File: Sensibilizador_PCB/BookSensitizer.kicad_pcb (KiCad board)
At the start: 2 copper layers, 70 x 57 mm, 40 parts, among them J3 Conn_inputs, M1 Fan, Q1 IRF630, Q2 IRF630, Q3 IRF630, Q4 IRF630, Q5 SI2302, T1 MountingHole_3.2mm_M3, T2 MountingHole_3.2mm_M3, T3 MountingHole_3.2mm_M3, U1 LM5104M, U2 LM5104M

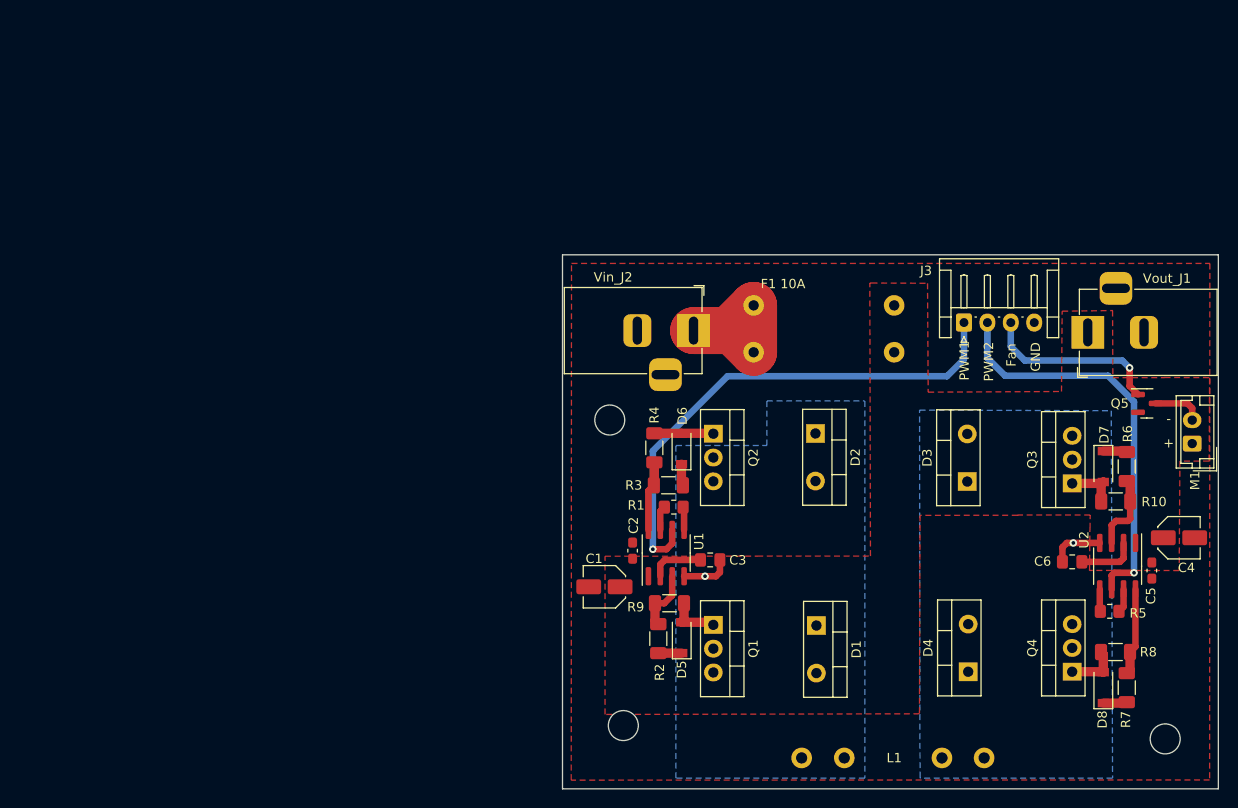
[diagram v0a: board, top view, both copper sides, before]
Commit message: mini arreglo para conectar una tierra
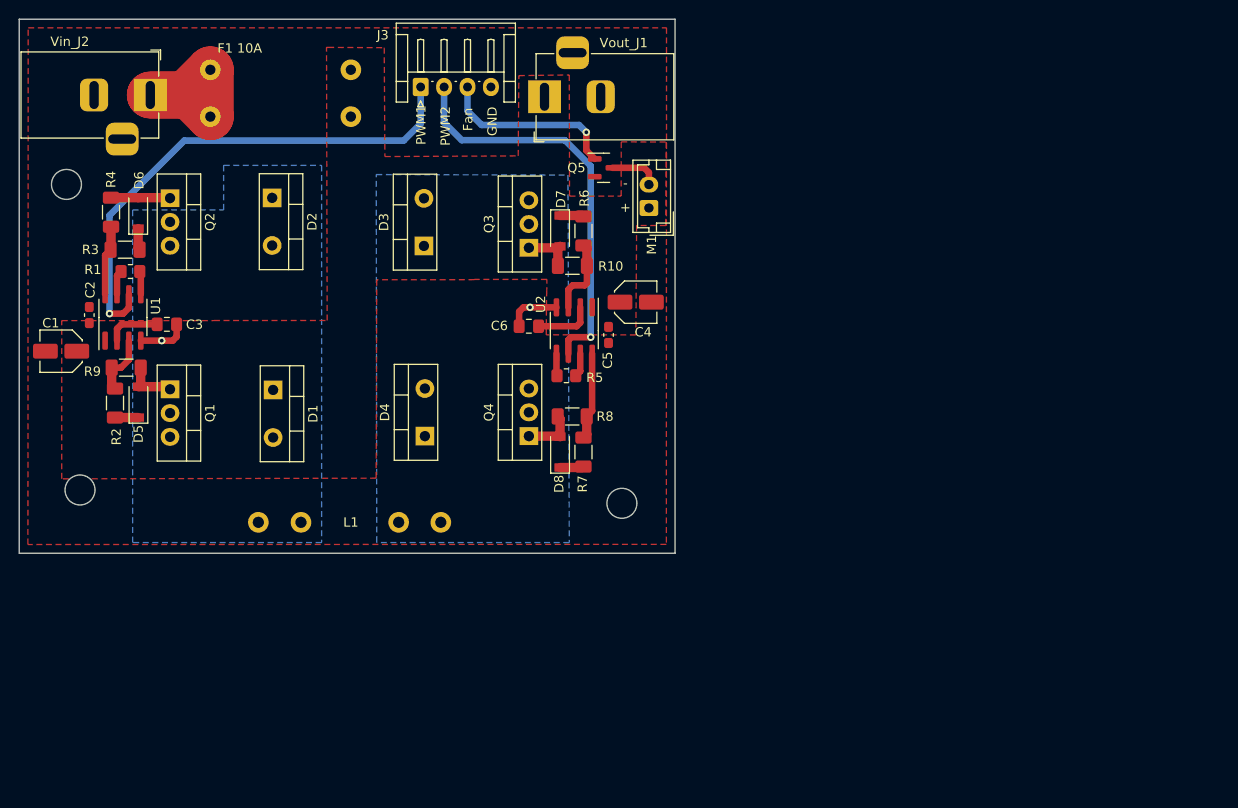
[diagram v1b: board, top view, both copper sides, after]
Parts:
- moved M1 63.2 mm to (118.1, 65.2)
- moved C2 63.2 mm to (58.4, 76.6)
- moved C3 63.2 mm to (66.7, 77.6)
- moved C5 63.2 mm to (113.8, 78.8)
- moved C6 63.2 mm to (105.3, 77.8)
- moved D1 63.2 mm to (78.0, 84.6)
- moved D2 63.2 mm to (77.9, 64.1)
- moved D7 63.2 mm to (108.6, 67.7)
- moved D8 63.2 mm to (108.6, 91.3)
- moved F1 10A 63.2 mm to (78.8, 53.0)
- moved J3 63.2 mm to (93.8, 52.3)
- moved Q1 63.2 mm to (67.0, 84.6)
- moved Q2 63.2 mm to (67.0, 64.2)
- moved Q3 63.2 mm to (105.3, 69.5)
- moved Q4 63.2 mm to (105.3, 89.6)
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
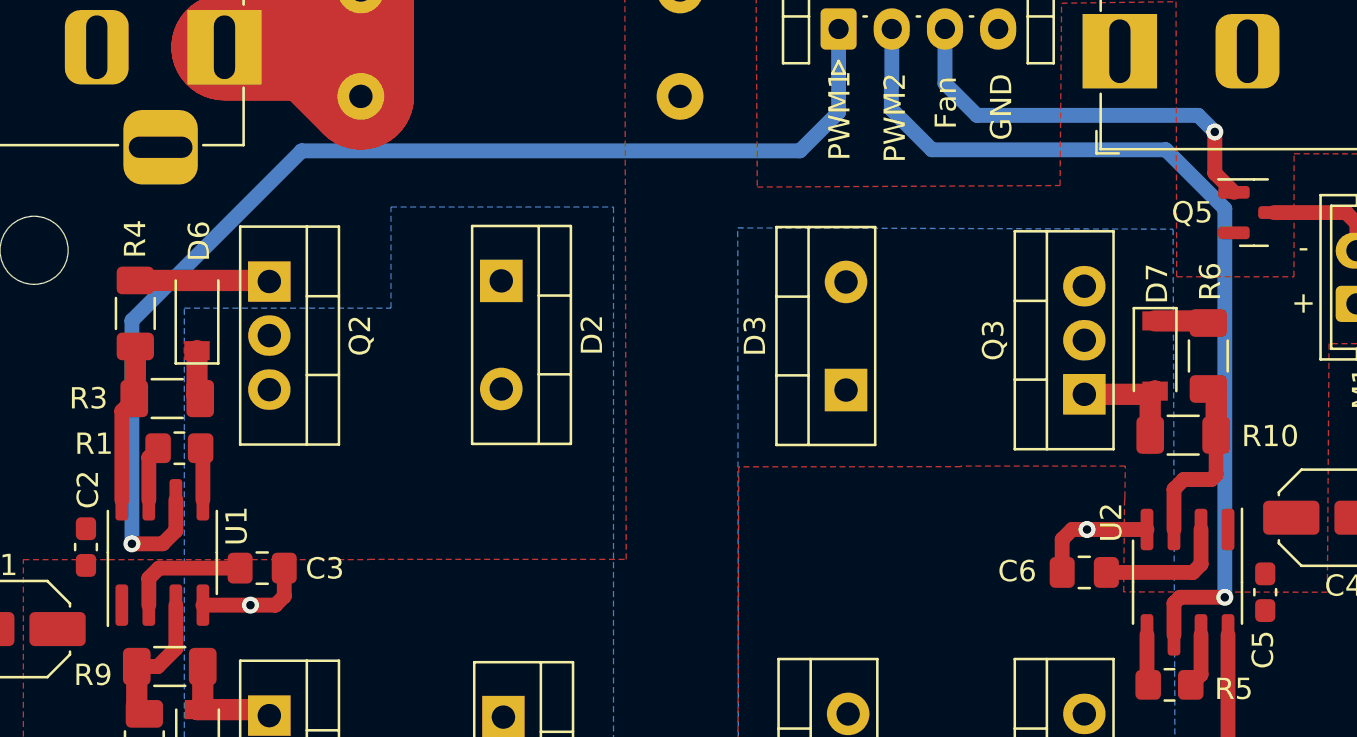
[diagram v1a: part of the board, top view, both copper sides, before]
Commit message: placa terminada
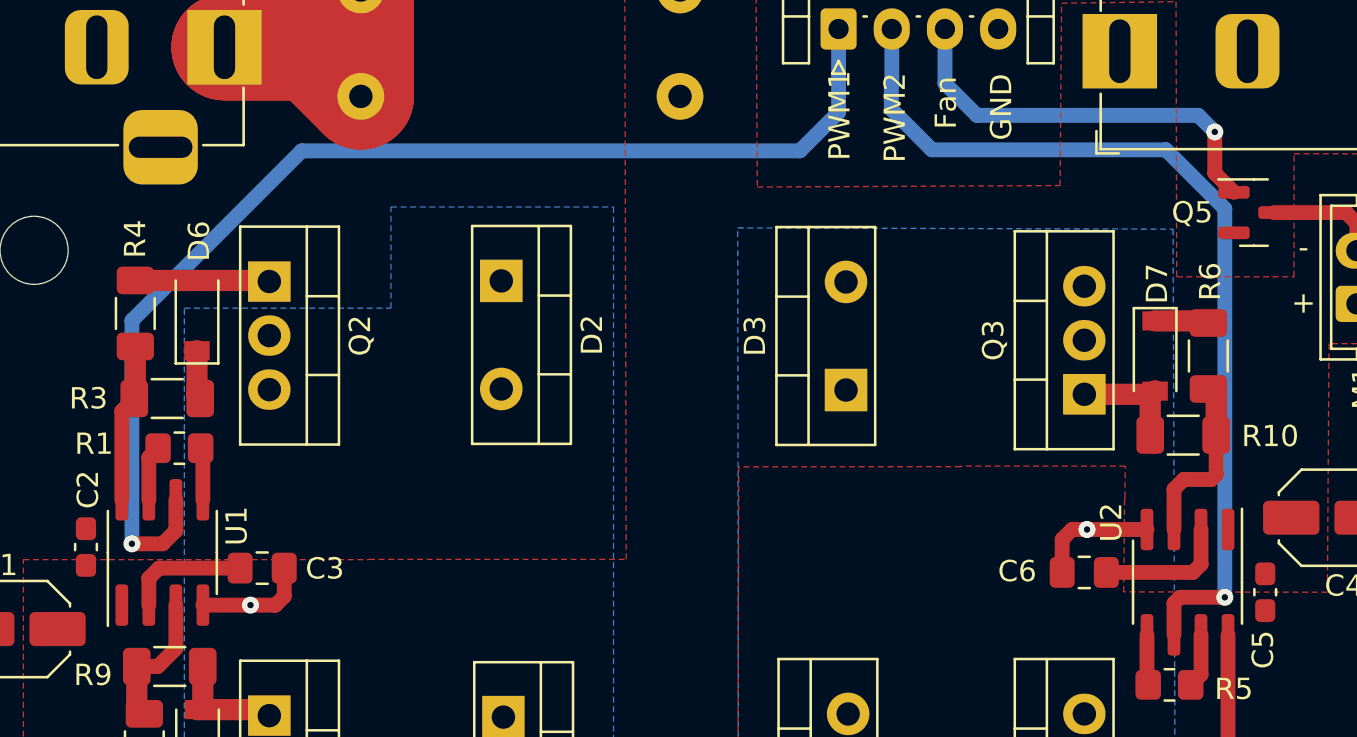
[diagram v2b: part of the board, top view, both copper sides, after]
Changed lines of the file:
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@@
   (segment (start 66.1242 79.3616) (end 67.298 79.3616) (width 0.7) (layer "F.Cu") (net 4))
   (segment (start 67.298 79.3616) (end 67.7125 78.9471) (width 0.7) (layer "F.Cu") (net 4))
-  (via (at 66.1242 79.3616) (size 0.8) (drill 0.4) (layers "F.Cu" "B.Cu") (net 4))
+  (via (at 66.1242 79.3616) (size 0.8) (drill 0.3) (layers "F.Cu" "B.Cu") (net 4))
   (segment (start 110.4138 77.8256) (end 106.3459 77.8256) (width 0.7) (layer "F.Cu") (net 5))
   (segment (start 110.7948 75.8078) (end 110.7948 77.4446) (width 0.7) (layer "F.Cu") (net 5))
@@
   (segment (start 105.438 75.8078) (end 108.2548 75.8078) (width 0.7) (layer "F.Cu") (net 6))
   (segment (start 104.2709 76.2723) (end 104.7354 75.8078) (width 0.7) (layer "F.Cu") (net 6))
-  (via (at 105.438 75.8078) (size 0.8) (drill 0.4) (layers "F.Cu" "B.Cu") (net 6))
+  (via (at 105.438 75.8078) (size 0.8) (drill 0.3) (layers "F.Cu" "B.Cu") (net 6))
   (segment (start 63.6372 87.5718) (end 61.1372 87.5718) (width 1) (layer "F.Cu") (net 7))
   (segment (start 108.4066 71.374) (end 108.4066 69.5342) (width 1) (layer "F.Cu") (net 8))
@@
   (segment (start 62.6182 74.4116) (end 62.6182 75.8626) (width 0.7) (layer "F.Cu") (net 13))
   (segment (start 62.6182 75.8626) (end 62.0014 76.4794) (width 0.7) (layer "F.Cu") (net 13))
-  (via (at 60.5536 76.4794) (size 0.8) (drill 0.4) (layers "F.Cu" "B.Cu") (net 13))
+  (via (at 60.5536 76.4794) (size 0.8) (drill 0.3) (layers "F.Cu" "B.Cu") (net 13))
   (segment (start 91.948 58.0136) (end 93.7618 56.1998) (width 0.7) (layer "B.Cu") (net 13))
   (segment (start 68.5292 58.0136) (end 91.948 58.0136) (width 0.7) (layer "B.Cu") (net 13))
@@
   (segment (start 109.5248 79.2734) (end 109.5248 80.7578) (width 0.7) (layer "F.Cu") (net 14))
   (segment (start 111.9124 78.994) (end 109.8042 78.994) (width 0.7) (layer "F.Cu") (net 14))
-  (via (at 111.9124 78.994) (size 0.8) (drill 0.4) (layers "F.Cu" "B.Cu") (net 14))
+  (via (at 111.9124 78.994) (size 0.8) (drill 0.3) (layers "F.Cu" "B.Cu") (net 14))
   (segment (start 111.9124 60.7314) (end 111.9124 78.994) (width 0.7) (layer "B.Cu") (net 14))
   (segment (start 96.2618 54.9106) (end 96.2618 52.2865) (width 0.7) (layer "B.Cu") (net 14))
@@
   (segment (start 111.4418 59.0615) (end 112.3443 59.964) (width 0.7) (layer "F.Cu") (net 15))
   (segment (start 111.4418 57.124) (end 111.4418 59.0615) (width 0.7) (layer "F.Cu") (net 15))
-  (via (at 111.4418 57.124) (size 0.8) (drill 0.4) (layers "F.Cu" "B.Cu") (net 15))
+  (via (at 111.4418 57.124) (size 0.8) (drill 0.3) (layers "F.Cu" "B.Cu") (net 15))
   (segment (start 100.2618 56.344) (end 110.6618 56.344) (width 0.7) (layer "B.Cu") (net 15))
   (segment (start 110.6618 56.344) (end 111.4418 57.124) (width 0.7) (layer "B.Cu") (net 15))
